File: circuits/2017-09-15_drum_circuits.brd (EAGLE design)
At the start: 32 x 46 mm, 30 parts, among them IC2 MIC5225-5v, U2 ATMEGA328P_TQFP

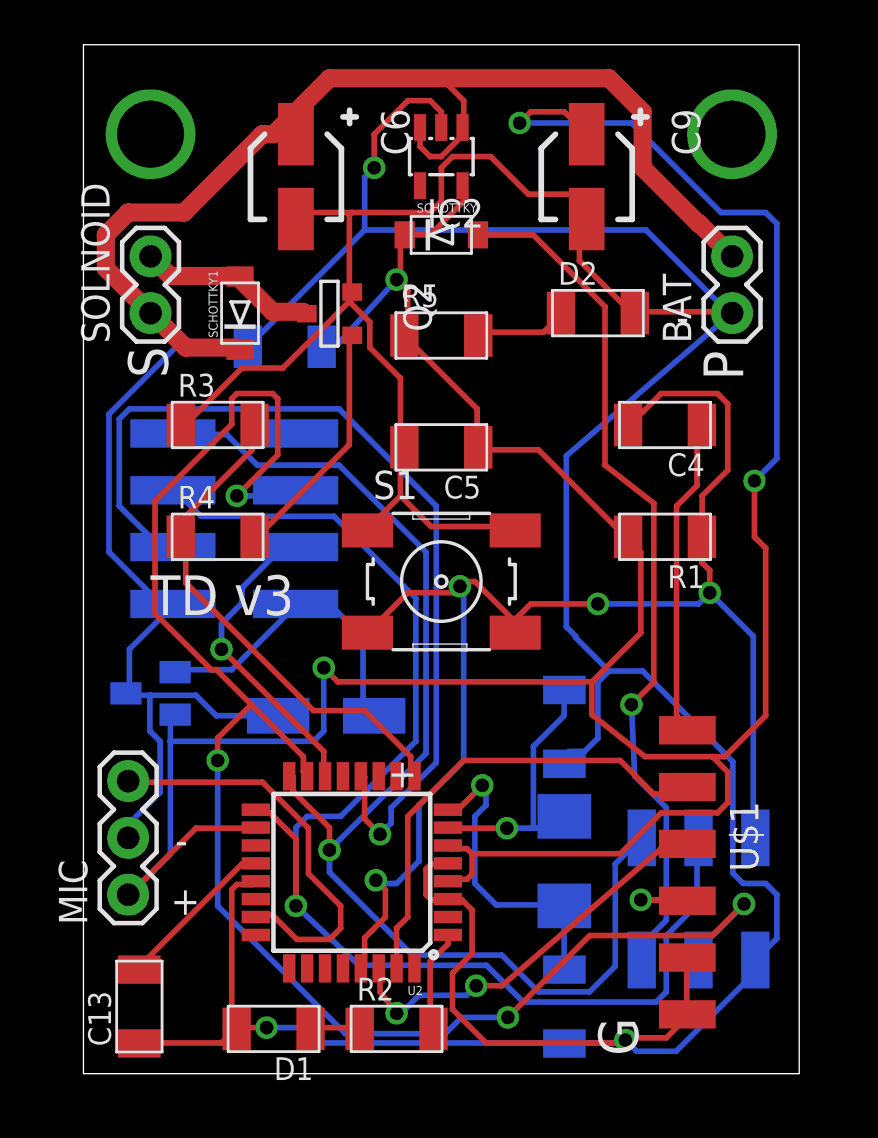
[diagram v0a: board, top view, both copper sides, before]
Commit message: clean
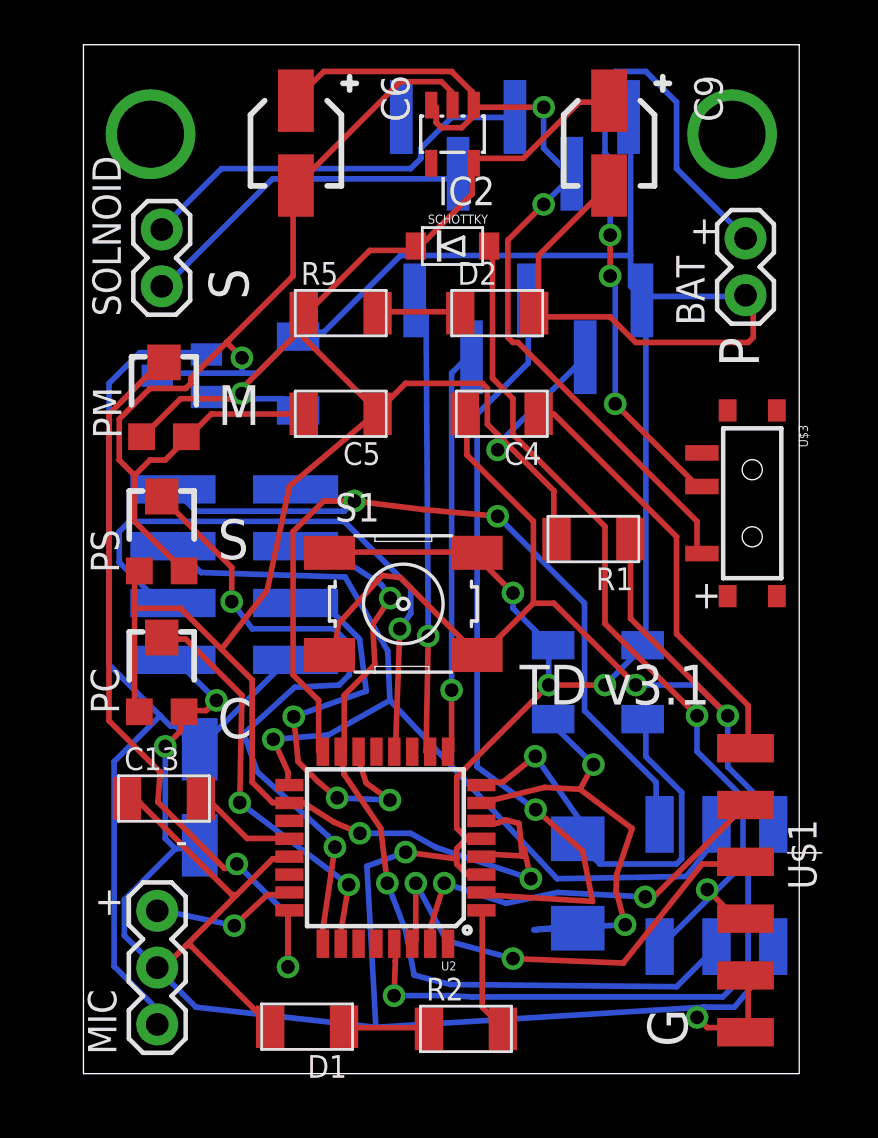
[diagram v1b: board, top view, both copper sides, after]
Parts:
- removed Q2: (no value), fab:SOT-23
- removed R3: 10k, fab:R1206FAB
- removed R4: 100, fab:R1206FAB
- removed SCHOTTKY1: (no value), adafruit:SOD-123FL
- added H_BRIDGE_INA, H_BRIDGE_OUT: (no value), pinhead-2:1X05SMD
- added PC, PM, PS: (no value), adafruit:TC33X
- added U$3: SWITCH_SPDT, SparkFun-Electromechanical:KPS-1290
- moved C2 14.9 mm to (25.0, 17.5), turned to 90 degrees
- moved VREG3.3 14.3 mm to (4.40, 31.2)
- moved C13 9.36 mm to (3.60, 12.3), turned to 0 degrees
- moved U$4 7.94 mm to (5.20, 14.5), turned to 180 degrees
- moved C4 7.32 mm to (18.7, 29.5)
- moved MIC 5.94 mm to (3.30, 2.20)
- moved C5 4.74 mm to (11.5, 29.5)
- moved R5 4.61 mm to (11.5, 34.0)
- moved D2 4.50 mm to (18.5, 34.0)
- moved R1 3.20 mm to (22.8, 23.9)
- moved R2 3.10 mm to (17.1, 2.00)
- moved U$1 2.72 mm to (29.6, 8.20)
- moved U$2 2.50 mm to (4.00, 18.5)
- moved C1 2.06 mm to (21.0, 17.5), turned to 90 degrees
- moved S1 1.97 mm to (14.3, 21.0)
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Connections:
- removed net DRAIN: Q2.1, SCHOTTKY1.A, SOLNOID.2
- removed net GATE_DO: R3.2, R4.1, U2.9
- removed net N$11: Q2.3, R4.2
- new net BAT_IN: BAT.2, U$3.P
- new net ENABLE: H_BRIDGE_INA.3, U2.2
- new net OUT: U$3.S
- new net PHASE: H_BRIDGE_INA.4, U2.9
- new net PM: PM.2, U2.24
- new net POT_C: PC.2, U2.26
- new net POT_S: PS.2, U2.25
- new net SLEEP: H_BRIDGE_INA.5, U2.10
- new net SOL_1: H_BRIDGE_OUT.4, SOLNOID.1
- new net SOL_2: H_BRIDGE_OUT.3, SOLNOID.2
- new net VM: H_BRIDGE_OUT.5
- net 3.3V: now also MIC.1
- net 5V: now also H_BRIDGE_INA.2, PC.1, PM.1, PS.1; no longer MIC.1
- net GND: now also H_BRIDGE_INA.1, H_BRIDGE_OUT.1, PC.3, PM.3, PS.3; no longer Q2.2, R3.1
- net VCC: now also H_BRIDGE_OUT.2, U$3.O; no longer BAT.2, SCHOTTKY1.C, SOLNOID.1
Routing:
- net ENABLE: track 0.00 -> 35.2 mm, vias 0 -> 1
- net MOSI: track 72.6 -> 37.9 mm, vias 4 -> 2
- net PM: track 0.00 -> 34.6 mm, vias 0 -> 2
- net 5V: track 143.7 -> 110.6 mm
- net BAT_IN: track 0.00 -> 31.3 mm, vias 0 -> 3
- net 3.3V: track 14.2 -> 44.7 mm
- net POT_S: track 0.00 -> 30.3 mm, vias 0 -> 2
- net GATE_DO: track 22.8 -> 0.00 mm
- net SCK: track 63.1 -> 41.5 mm
- net SLEEP: track 0.00 -> 20.6 mm, vias 0 -> 1
- net PHASE: track 0.00 -> 18.3 mm, vias 0 -> 1
- net POT_C: track 0.00 -> 18.2 mm, vias 0 -> 2
- net SOL_2: track 0.00 -> 18.2 mm
- net VCC: track 58.4 -> 41.5 mm, vias 0 -> 2
- net SOL_1: track 0.00 -> 15.4 mm
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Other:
- board text added: "C"
- board text added: "M"
- board text added: "TD v3.1"
- board text removed: "TD v3"
